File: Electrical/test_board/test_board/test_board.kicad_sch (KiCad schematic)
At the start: 31 parts, among them J1 Screw_Terminal_01x04, J10 Conn_01x06_Pin, J11 Conn_01x04_Socket, J12 Conn_01x06_Pin, J13 Conn_01x04_Socket, J2 Conn_01x06_Pin, J3 Conn_01x04_Socket, J4 Conn_01x06_Pin, J5 Conn_01x04_Socket, J6 Conn_01x06_Pin, J7 Conn_01x04_Socket, J8 Conn_01x06_Pin, J9 Conn_01x04_Socket

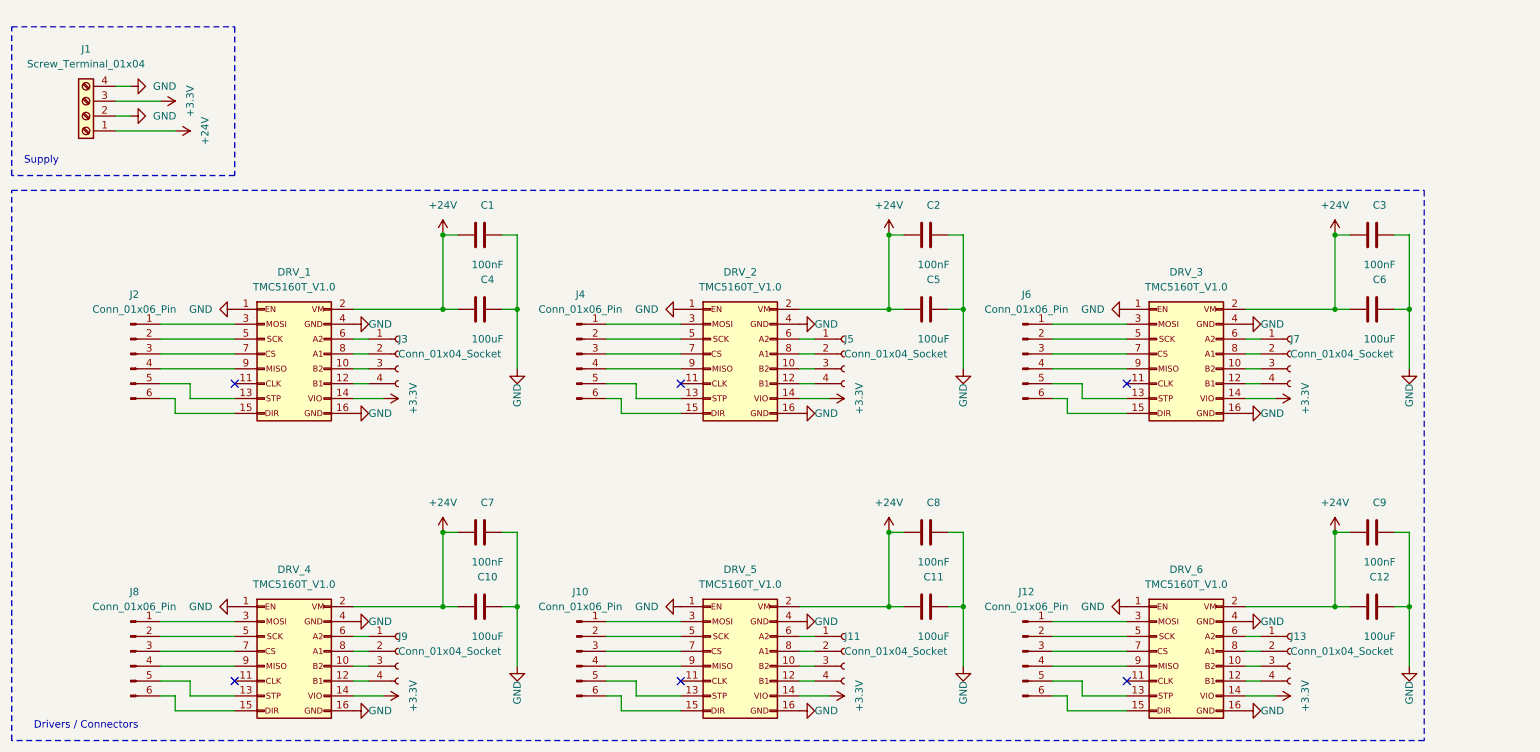
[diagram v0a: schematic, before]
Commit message: Fixed the whole test thing
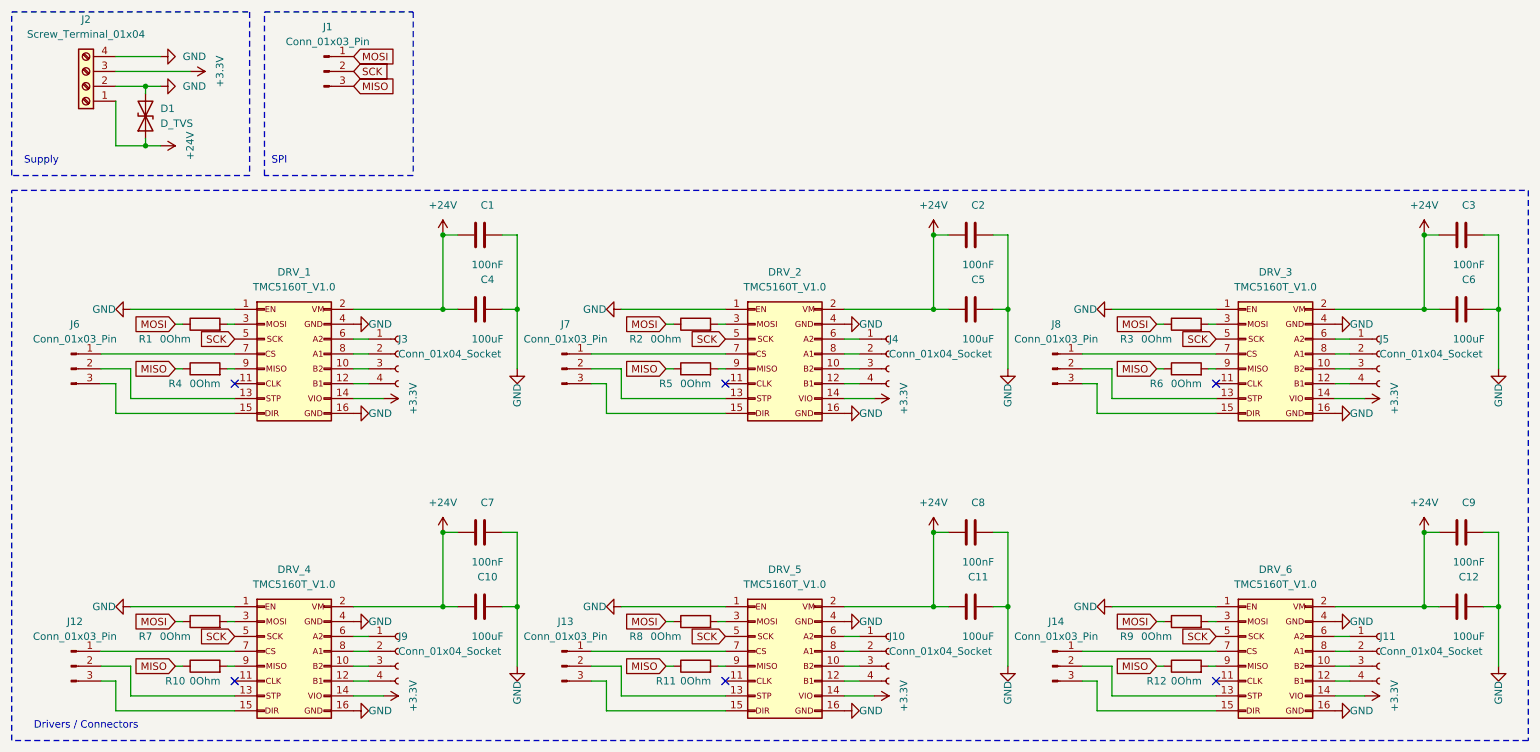
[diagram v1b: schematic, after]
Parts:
- removed J10, J12, J2, J4, J6, J8: Conn_01x06_Pin, Connector_PinHeader_2.54mm:PinHeader_1x06_P2.54mm_Vertical, symbol Connector:Conn_01x06_Pin
- added D1: D_TVS, Diode_THT:D_DO-201AD_P15.24mm_Horizontal, symbol Device:D_TVS
- added J1, J12, J13, J14, J6, J7, J8: Conn_01x03_Pin, Connector_PinHeader_2.54mm:PinHeader_1x03_P2.54mm_Vertical, symbol Connector:Conn_01x03_Pin
- added R1, R10, R11, R12, R2, R3, R4, R5, R6, R7, R8, R9: 0Ohm, Resistor_THT:R_Axial_DIN0207_L6.3mm_D2.5mm_P10.16mm_Horizontal, symbol Device:R
- renumbered J11 to J10, J13 to J11, J1 to J2, J5 to J4, J7 to J5
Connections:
- net +24V: now also D1.1 (A1)
- net GND: now also D1.2 (A2)
- net at DRV_2.3 (Pin_3): now also R2.2
- net SCK: now reaches DRV_2.5 (Pin_5)
- net SCK: now also DRV_1.5 (Pin_5), DRV_3.5 (Pin_5), DRV_4.5 (Pin_5), DRV_5.5 (Pin_5), DRV_6.5 (Pin_5), J1.2 (Pin_2)
- net at DRV_2.7 (Pin_7): now also J7.1 (Pin_1)
- net at DRV_2.9 (Pin_9): now also R5.2
- net at DRV_2.13 (Pin_13): now also J7.2 (Pin_2)
- net at DRV_2.15 (Pin_15): now also J7.3 (Pin_3)
- net at DRV_4.3 (Pin_3): now also R7.2
- net at DRV_4.7 (Pin_7): now also J12.1 (Pin_1)
- net at DRV_4.9 (Pin_9): now also R10.2
- net at DRV_4.13 (Pin_13): now also J12.2 (Pin_2)
- net at DRV_4.15 (Pin_15): now also J12.3 (Pin_3)
- net at DRV_3.3 (Pin_3): now also R3.2
- net at DRV_3.7 (Pin_7): now also J8.1 (Pin_1)
- net at DRV_3.9 (Pin_9): now also R6.2
- net at DRV_3.13 (Pin_13): now also J8.2 (Pin_2)
- net at DRV_3.15 (Pin_15): now also J8.3 (Pin_3)
- net at DRV_1.3 (Pin_3): now also R1.2
- net at DRV_1.7 (Pin_7): now also J6.1 (Pin_1)
- net at DRV_1.9 (Pin_9): now also R4.2
- net at DRV_1.13 (Pin_13): now also J6.2 (Pin_2)
- net at DRV_1.15 (Pin_15): now also J6.3 (Pin_3)
- net at DRV_6.3 (Pin_3): now also R9.2
- net at DRV_6.7 (Pin_7): now also J14.1 (Pin_1)
- net at DRV_6.9 (Pin_9): now also R12.2
- net at DRV_6.13 (Pin_13): now also J14.2 (Pin_2)
- net at DRV_6.15 (Pin_15): now also J14.3 (Pin_3)
- net at DRV_5.3 (Pin_3): now also R8.2
- net at DRV_5.7 (Pin_7): now also J13.1 (Pin_1)
- net at DRV_5.9 (Pin_9): now also R11.2
- net at DRV_5.13 (Pin_13): now also J13.2 (Pin_2)
- net at DRV_5.15 (Pin_15): now also J13.3 (Pin_3)
- new net MISO: J1.3 (Pin_3), R10.1, R11.1, R12.1, R4.1, R5.1, R6.1
- new net MOSI: J1.1 (Pin_1), R1.1, R2.1, R3.1, R7.1, R8.1, R9.1
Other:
- note added: "SPI"
- moved on the sheet: C11, C12, C2, C3, C5, C6, C8, C9, DRV_2, DRV_3, DRV_5, DRV_6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
